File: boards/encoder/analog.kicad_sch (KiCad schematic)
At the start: 26 parts, among them Q1 Q_PMOS_GSD, U10 QSZ2TR, U3 CT310, U4 INA826, U5 INA826, U6 LMR342FVJ, U7 AZ431-A

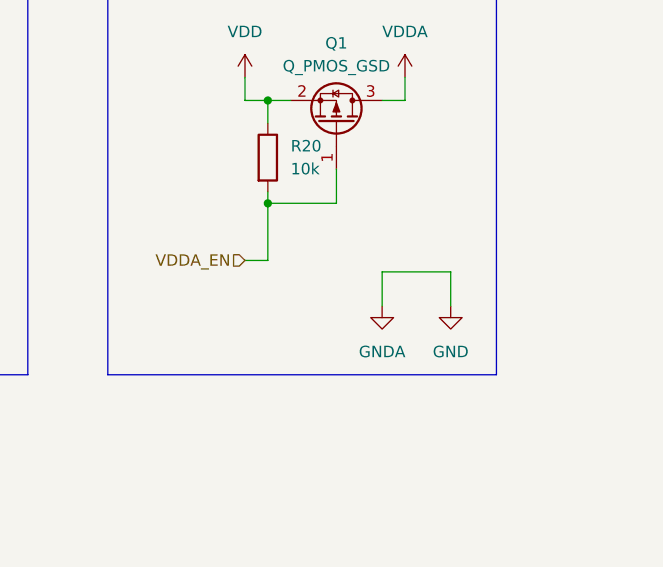
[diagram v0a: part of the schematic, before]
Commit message: v0.2.7
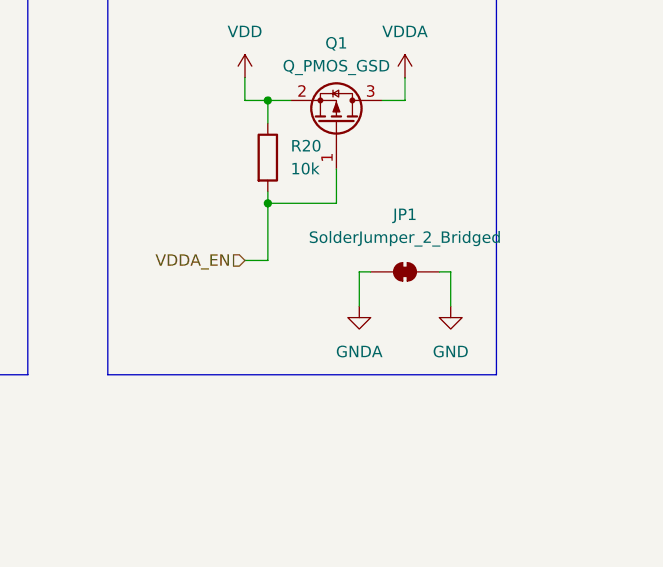
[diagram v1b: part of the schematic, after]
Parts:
- added JP1: SolderJumper_2_Bridged, Jumper:SolderJumper-2_P1.3mm_Bridged_Pad1.0x1.5mm, symbol Jumper:SolderJumper_2_Bridged
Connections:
- net GND: now also JP1.2 (B); no longer C10.2, C11.2, C12.2, C5.2, C6.2, C7.2, C8.1, C9.1, R21.1, U10.5 (CP), U3.4 (GSIN), U3.8 (GCOS), U3.9 (EP), U4.5 (GND), U4.9 (EP), U5.5 (GND), U5.9 (EP), U6.4 (V-), U7.3 (A)
- new net GNDA: C10.2, C11.2, C12.2, C5.2, C6.2, C7.2, C8.1, C9.1, JP1.1 (A), R21.1, U10.5 (CP), U3.4 (GSIN), U3.8 (GCOS), U3.9 (EP), U4.5 (GND), U4.9 (EP), U5.5 (GND), U5.9 (EP), U6.4 (V-), U7.3 (A)
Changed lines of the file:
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@@
 	(wire
 		(pts
-			(xy 224.79 105.41) (xy 217.17 105.41)
-		)
-		(stroke
-			(width 0)
-			(type default)
-		)
-	)
-	(wire
-		(pts
 			(xy 31.75 44.45) (xy 31.75 46.99)
 		)
@@
 	(wire
 		(pts
+			(xy 214.63 105.41) (xy 215.9 105.41)
+		)
+		(stroke
+			(width 0)
+			(type default)
+		)
+	)
+	(wire
+		(pts
 			(xy 106.68 102.87) (xy 106.68 106.68)
 		)
@@
 	(wire
 		(pts
+			(xy 223.52 105.41) (xy 224.79 105.41)
+		)
+		(stroke
+			(width 0)
+			(type default)
+		)
+	)
+	(wire
+		(pts
 			(xy 143.51 41.91) (xy 147.32 41.91)
 		)
@@
 	(wire
 		(pts
-			(xy 217.17 105.41) (xy 217.17 109.22)
+			(xy 214.63 105.41) (xy 214.63 109.22)
 		)
 		(stroke
@@
 	(symbol
 		(lib_id "power:GNDA")
-		(at 217.17 109.22 0)
+		(at 214.63 109.22 0)
 		(unit 1)
 		(exclude_from_sim no)
@@
 		(fields_autoplaced yes)
 		(property "Reference" "#PWR050"
-			(at 217.17 115.57 0)
+			(at 214.63 115.57 0)
 			(effects
 				(font
@@
 		)
 		(property "Value" "GNDA"
-			(at 217.17 114.3 0)
+			(at 214.63 114.3 0)
 			(effects
 				(font
@@
 		)
 		(property "Footprint" ""
-			(at 217.17 109.22 0)
+			(at 214.63 109.22 0)
 			(effects
 				(font
@@
 		)
 		(property "Datasheet" ""
-			(at 217.17 109.22 0)
+			(at 214.63 109.22 0)
 			(effects
 				(font
@@
 		)
 		(property "Description" "Power symbol creates a global label with name \"GNDA\" , analog ground"
-			(at 217.17 109.22 0)
+			(at 214.63 109.22 0)
 			(effects
 				(font
@@
 					(unit 1)
 				)
+			)
+		)
+	)
+	(symbol
+		(lib_id "Jumper:SolderJumper_2_Bridged")
+		(at 219.71 105.41 0)
+		(unit 1)
+		(exclude_from_sim no)
+		(in_bom no)
+		(on_board yes)
+		(dnp no)
+		(fields_autoplaced yes)
+		(property "Reference" "JP1"
+			(at 219.71 99.06 0)
+			(effects
+				(font
+					(size 1.27 1.27)
+				)
+			)
+		)
+		(property "Value" "SolderJumper_2_Bridged"
+			(at 219.71 101.6 0)
+			(effects
+				(font
+					(size 1.27 1.27)
+				)
+			)
+		)
+		(property "Footprint" "Jumper:SolderJumper-2_P1.3mm_Bridged_Pad1.0x1.5mm"
+			(at 219.71 105.41 0)
+			(effects
+				(font
+					(size 1.27 1.27)
+				)
+				(hide yes)
+			)
+		)
+		(property "Datasheet" "~"
+			(at 219.71 105.41 0)
+			(effects
+				(font
+					(size 1.27 1.27)
+				)
+				(hide yes)
+			)
+		)
+		(property "Description" "Solder Jumper, 2-pole, closed/bridged"
+			(at 219.71 105.41 0)
+			(effects
+				(font
+					(size 1.27 1.27)
+				)
+				(hide yes)
+			)
+		)
+		(pin "1"
+		)
+		(pin "2"
+		)
+		(instances
+			(project ""
+				(path "/710faa81-ee23-422b-ba7e-b655a364ab6f/763a463a-636e-4b92-a93e-dd97da54b348"
+					(reference "JP1")
+					(unit 1)
+				)
